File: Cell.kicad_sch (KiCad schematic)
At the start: 20 parts

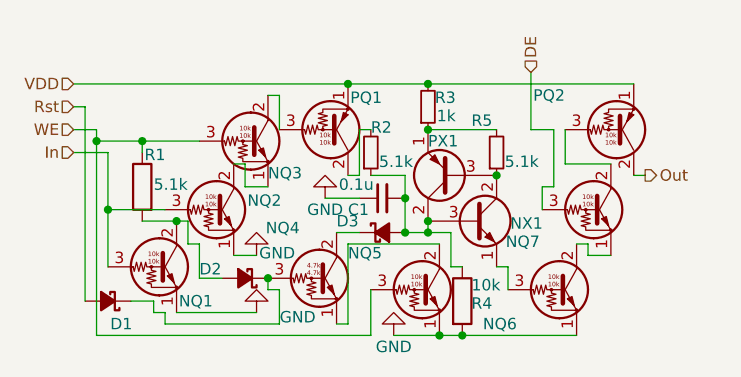
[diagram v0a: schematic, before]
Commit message: Remaking due to design change, wip1
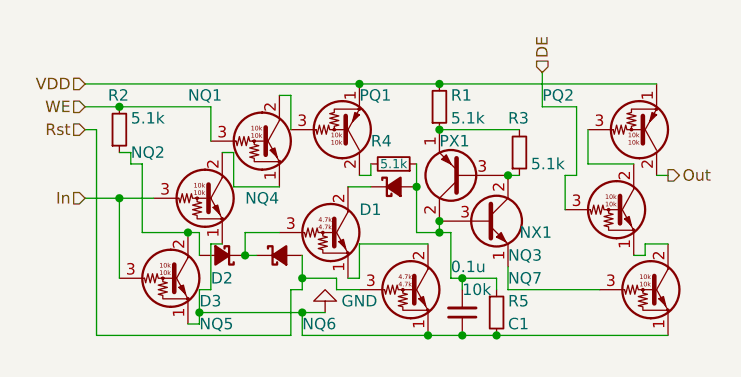
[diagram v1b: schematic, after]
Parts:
- removed NQ6: DTC114E-THT, Package_TO_SOT_THT:TO-92_Inline_Wide, symbol YoshLibrary:DTC114E-THT
- removed R1: 5.1k, YoshLibrary:R_Axial_DIN0207_L6.3mm_D2.5mm_P7.62mm_Horizontal_Y, symbol Device:R
- removed R4: 10k, YoshLibrary:R_Axial_DIN0207_L6.3mm_D2.5mm_P7.62mm_Horizontal_Y, symbol Device:R
- added NQ6: DTC143E-THT, Package_TO_SOT_THT:TO-92_Inline_Wide, symbol YoshLibrary:DTC143E-THT
- added R1, R4: 5.1k, Resistor_THT:R_Axial_DIN0207_L6.3mm_D2.5mm_P7.62mm_Horizontal, symbol Device:R_Small
- D1, D2, D3: value Schottky -> 30V0.2A
- R2: footprint YoshLibrary:R_Axial_DIN0207_L6.3mm_D2.5mm_P7.62mm_Horizontal_Y -> Resistor_THT:R_Axial_DIN0207_L6.3mm_D2.5mm_P7.62mm_Horizontal
- R3: value 1k -> 5.1k; footprint YoshLibrary:R_Axial_DIN0207_L6.3mm_D2.5mm_P7.62mm_Horizontal_Y -> Resistor_THT:R_Axial_DIN0207_L6.3mm_D2.5mm_P7.62mm_Horizontal
- R5: value 5.1k -> 10k; footprint YoshLibrary:R_Axial_DIN0207_L6.3mm_D2.5mm_P7.62mm_Horizontal_Y -> Resistor_THT:R_Axial_DIN0207_L6.3mm_D2.5mm_P7.62mm_Horizontal
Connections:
- net DE: now also NQ3.3 (B); no longer NQ7.3 (B)
- net GND: now also NQ7.1 (E), R5.2, NQ6.1 (E); no longer NQ1.1 (E)
- net In: now also NQ5.3 (B); no longer NQ1.3 (B)
- net Rst: now also D3.2 (A), NQ6.3 (B); no longer D1.2 (A)
- net VDD: now also R1.2; no longer R3.2
- net WE: now also NQ1.3 (B), R2.2; no longer NQ3.3 (B), NQ5.3 (B)
- net at NQ4.2 (C): now also D1.1 (K); no longer D3.1 (K)
- net at C1.2, NX1.3 (B), PX1.2 (C): now also D1.2 (A), R5.1, R4.1; no longer D3.2 (A), R2.1
- net at D2.2 (A): now also NQ5.2 (C), R2.1; no longer NQ1.2 (C)
- net at NQ3.1 (E): now also NQ7.2 (C); no longer NQ2.2 (C)
- net at NQ4.1 (E): now also NQ6.2 (C); no longer NQ5.2 (C)
- net at D2.1 (K), NQ4.3 (B): now also D3.1 (K); no longer D1.1 (K)
- net at NQ3.2 (C): now also PQ2.3 (B); no longer PQ1.3 (B)
- net at NX1.1 (E): now also NQ7.3 (B)
- net at NX1.2 (C), PX1.3 (B): now also R3.1; no longer R5.1
- net at PQ1.2 (C): now also R4.2; no longer R2.2
- new net: NQ1.2 (C), PQ1.3 (B)
- new net: NQ1.1 (E), NQ2.2 (C)
- new net: PX1.1 (E), R1.1, R3.2

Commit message: New design completed
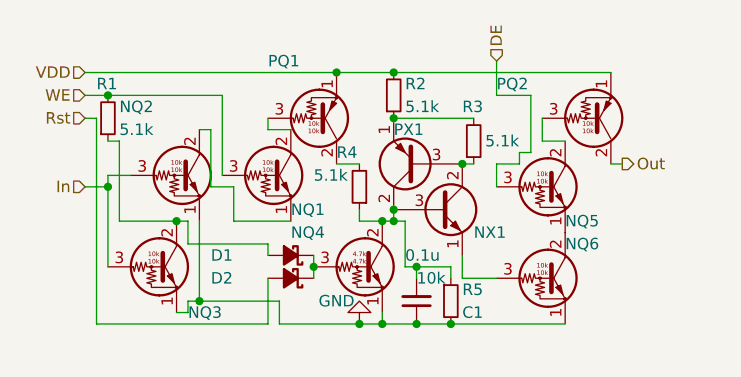
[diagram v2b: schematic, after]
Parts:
- removed D1: 30V0.2A, Diode_THT:D_DO-35_SOD27_P7.62mm_Horizontal, symbol Device:D_Schottky_Small_Filled
- removed NQ6: DTC143E-THT, Package_TO_SOT_THT:TO-92_Inline_Wide, symbol YoshLibrary:DTC143E-THT
- renumbered D2 to D1, D3 to D2, NQ5 to NQ3, NQ3 to NQ5, NQ7 to NQ6, R2 to R1, R1 to R2
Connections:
- net GND: now also NQ4.1 (E)
- net at NQ4.2 (C): now also C1.2, NX1.3 (B), PX1.2 (C), R4.1, R5.1
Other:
- moved on the sheet: C1, D1, D2, NQ1, NQ2, NQ3, NQ4, NQ5, NQ6, NX1, PQ1, PQ2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
